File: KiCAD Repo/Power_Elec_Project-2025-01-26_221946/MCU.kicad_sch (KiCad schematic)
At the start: 1 part, among them U2 LAUNCHXL-F28379D

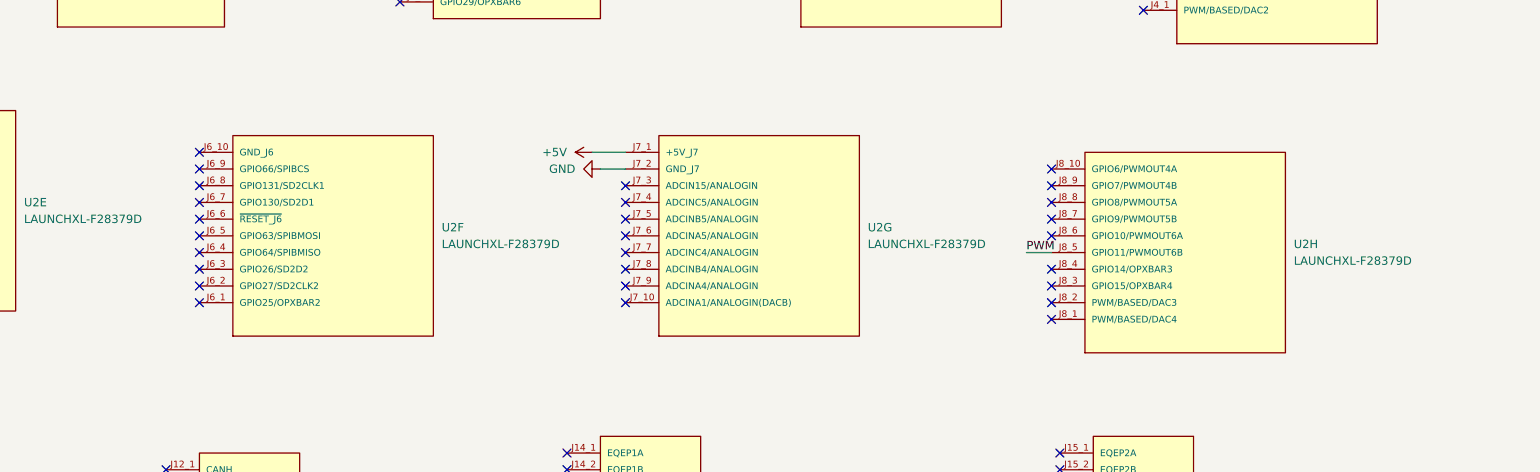
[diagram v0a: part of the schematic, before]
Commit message: PCB fix
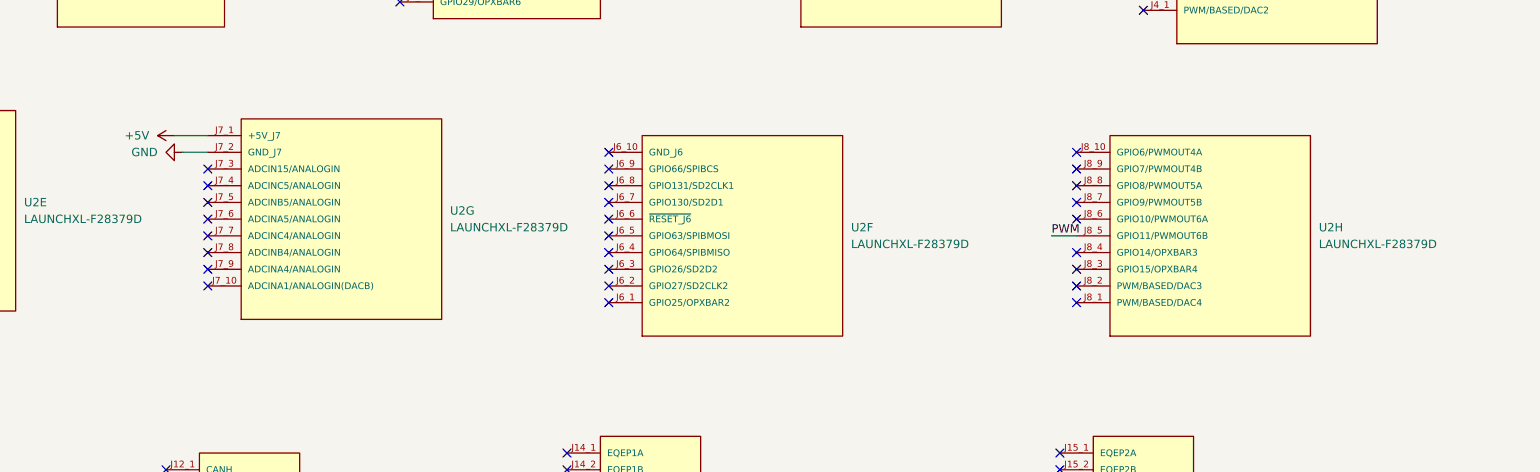
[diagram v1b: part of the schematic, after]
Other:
- moved on the sheet: U2F, U2G, U2H
